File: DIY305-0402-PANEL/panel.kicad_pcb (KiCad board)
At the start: 2 copper layers, 45.2 x 39 mm, 388 parts, among them J1 Conn_01x07, J2 Conn_01x07

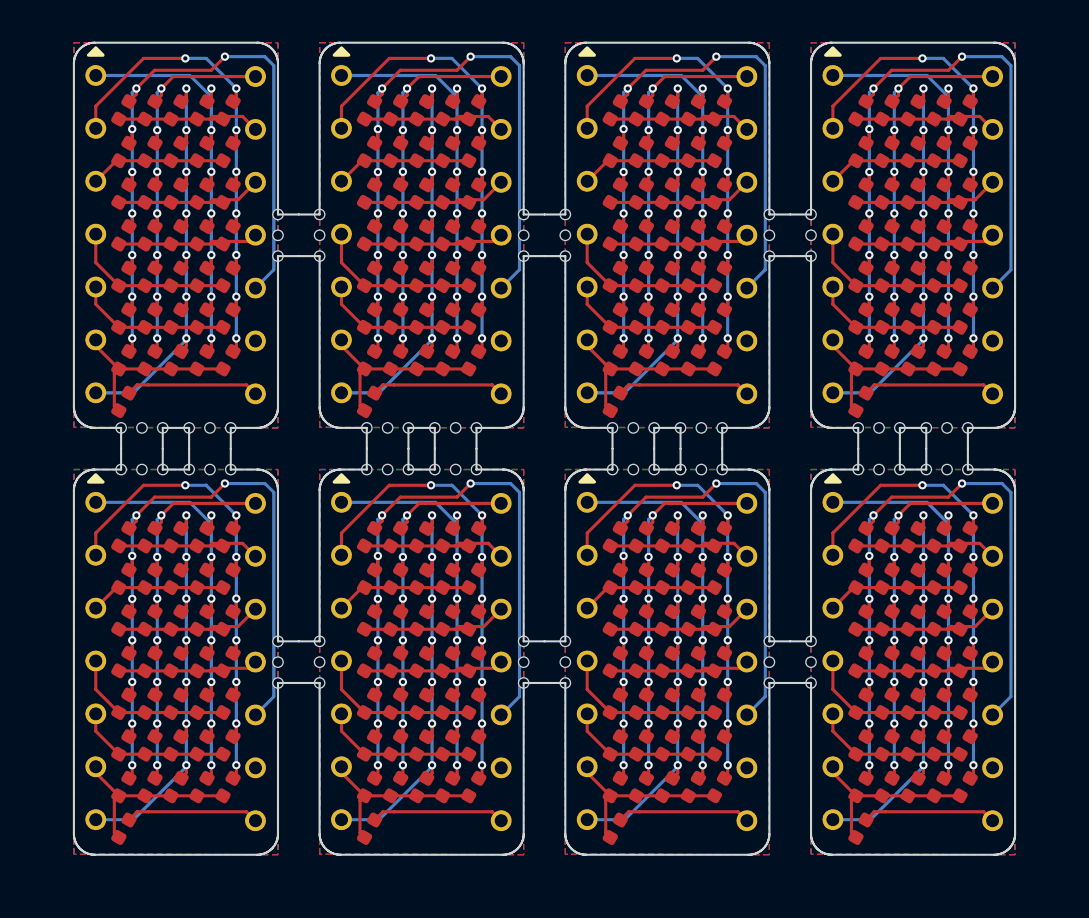
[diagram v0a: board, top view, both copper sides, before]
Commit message: Added pannel
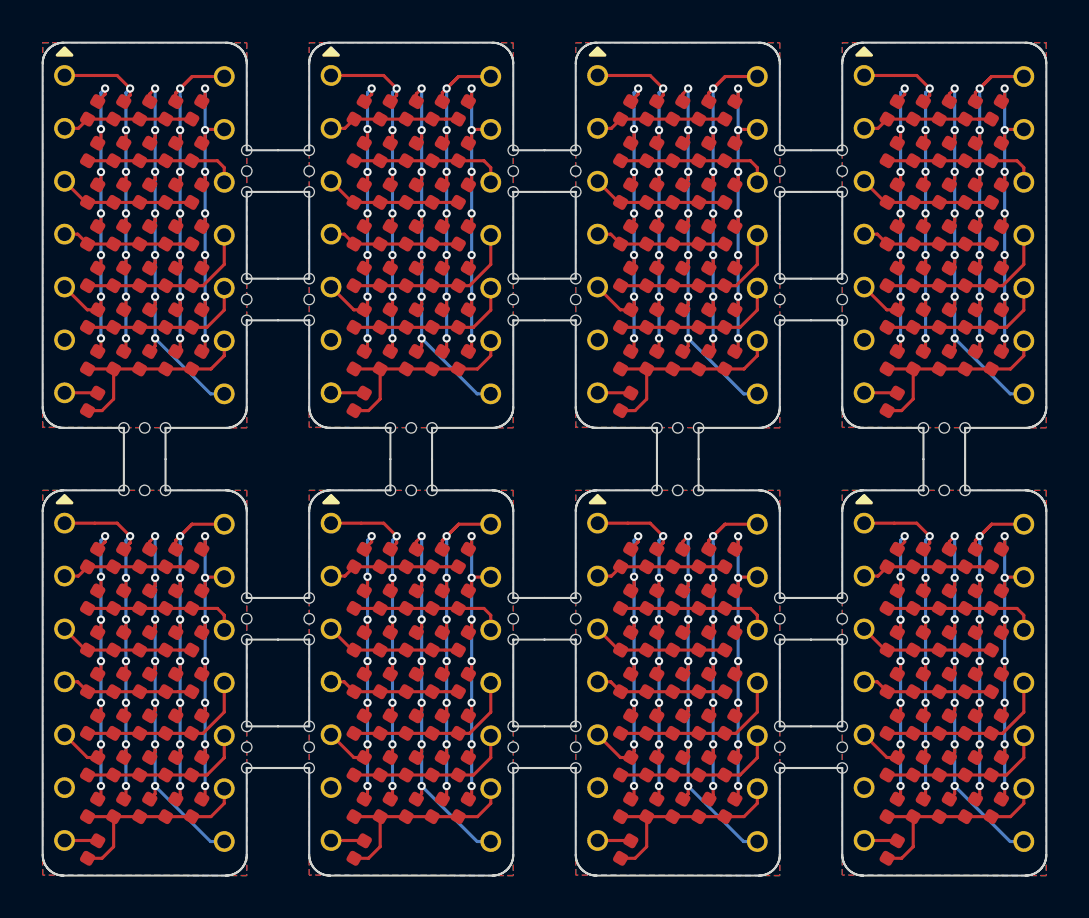
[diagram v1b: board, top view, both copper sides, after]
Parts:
- removed the D1 at (128.3, 23.2)
- removed the D1 at (128.3, 43.8)
- removed the D1 at (140.1, 23.2)
- removed the D1 at (151.9, 23.2)
- removed the D1 at (163.7, 43.8)
- removed the D1 at (163.7, 23.2)
- removed the D1 at (140.1, 43.8)
- removed the D1 at (151.9, 43.8)
- removed the D10 at (141.3, 27.2)
- removed the D10 at (164.9, 47.8)
- removed the D10 at (129.6, 47.8)
- removed the D10 at (129.6, 27.2)
- removed the D10 at (153.2, 27.2)
- removed the D10 at (153.2, 47.8)
- removed the D10 at (141.3, 47.8)
- removed the D10 at (164.9, 27.2)
- removed the D11 at (153.2, 29.2)
- removed the D11 at (129.6, 49.8)
- removed the D11 at (153.2, 49.8)
- removed the D11 at (141.3, 49.8)
- removed the D11 at (141.3, 29.2)
- removed the D11 at (164.9, 29.2)
- removed the D11 at (164.9, 49.8)
- removed the D11 at (129.6, 29.2)
- removed the D12 at (153.2, 31.2)
- removed the D12 at (164.9, 31.2)
- removed the D12 at (141.3, 31.2)
- removed the D12 at (129.6, 51.8)
- removed the D12 at (164.9, 51.8)
- removed the D12 at (129.6, 31.2)
- removed the D12 at (153.2, 51.8)
- removed the D12 at (141.3, 51.8)
- removed the D13 at (141.3, 33.2)
- removed the D13 at (164.9, 53.8)
- removed the D13 at (164.9, 33.2)
- removed the D13 at (129.6, 53.8)
- removed the D13 at (141.3, 53.8)
- removed the D13 at (153.2, 53.8)
- removed the D13 at (153.2, 33.2)
- removed the D13 at (129.6, 33.2)
- removed the D14 at (164.9, 55.8)
- removed the D14 at (164.9, 35.2)
- removed the D14 at (153.2, 35.2)
- removed the D14 at (141.3, 35.2)
- removed the D14 at (129.6, 55.8)
- removed the D14 at (129.6, 35.2)
- removed the D14 at (141.3, 55.8)
- removed the D14 at (153.2, 55.8)
- removed the D15 at (130.8, 23.2)
- removed the D15 at (166.2, 43.8)
- removed the D15 at (130.8, 43.8)
- removed the D15 at (166.2, 23.2)
- removed the D15 at (154.4, 43.8)
- removed the D15 at (142.6, 43.8)
- removed the D15 at (154.4, 23.2)
- removed the D15 at (142.6, 23.2)
- removed the D16 at (142.6, 25.2)
- removed the D16 at (154.4, 25.2)
- removed the D16 at (166.2, 45.8)
- removed the D16 at (142.6, 45.8)
- removed the D16 at (166.2, 25.2)
- removed the D16 at (130.8, 45.8)
- removed the D16 at (130.8, 25.2)
- removed the D16 at (154.4, 45.8)
- removed the D17 at (142.6, 47.8)
- removed the D17 at (130.8, 47.8)
- removed the D17 at (130.8, 27.2)
- removed the D17 at (154.4, 47.8)
- removed the D17 at (154.4, 27.2)
- removed the D17 at (166.2, 27.2)
- removed the D17 at (166.2, 47.8)
- removed the D17 at (142.6, 27.2)
- removed the D18 at (154.4, 29.2)
- removed the D18 at (142.6, 29.2)
- removed the D18 at (154.4, 49.8)
- removed the D18 at (166.2, 29.2)
- removed the D18 at (130.8, 29.2)
- removed the D18 at (166.2, 49.8)
- removed the D18 at (130.8, 49.8)
- removed the D18 at (142.6, 49.8)
- removed the D19 at (166.2, 31.2)
- removed the D19 at (154.4, 31.2)
- removed the D19 at (154.4, 51.8)
- removed the D19 at (142.6, 31.2)
- removed the D19 at (130.8, 51.8)
- removed the D19 at (130.8, 31.2)
- removed the D19 at (166.2, 51.8)
- removed the D19 at (142.6, 51.8)
- removed the D2 at (151.9, 45.8)
- removed the D2 at (128.3, 45.8)
- removed the D2 at (163.7, 45.8)
- removed the D2 at (163.7, 25.2)
- removed the D2 at (140.1, 25.2)
- removed the D2 at (140.1, 45.8)
- removed the D2 at (151.9, 25.2)
- removed the D2 at (128.3, 25.2)
- removed the D20 at (154.4, 33.2)
- removed the D20 at (166.2, 33.2)
- removed the D20 at (142.6, 53.8)
- removed the D20 at (130.8, 53.8)
- removed the D20 at (154.4, 53.8)
- removed the D20 at (130.8, 33.2)
- removed the D20 at (166.2, 53.8)
- removed the D20 at (142.6, 33.2)
- removed the D21 at (142.6, 35.2)
- removed the D21 at (166.2, 35.2)
- removed the D21 at (166.2, 55.8)
- removed the D21 at (154.4, 35.2)
- removed the D21 at (130.8, 55.8)
- removed the D21 at (154.4, 55.8)
- removed the D21 at (130.8, 35.2)
- removed the D21 at (142.6, 55.8)
- removed the D22 at (143.8, 43.8)
- removed the D22 at (143.8, 23.2)
- removed the D22 at (132.1, 43.8)
- removed the D22 at (167.4, 23.2)
- removed the D22 at (155.7, 43.8)
- removed the D22 at (155.7, 23.2)
- removed the D22 at (132.1, 23.2)
- removed the D22 at (167.4, 43.8)
- removed the D23 at (132.1, 45.8)
- removed the D23 at (167.4, 25.2)
- removed the D23 at (132.1, 25.2)
- removed the D23 at (155.7, 45.8)
- removed the D23 at (155.7, 25.2)
- removed the D23 at (143.8, 45.8)
- removed the D23 at (143.8, 25.2)
- removed the D23 at (167.4, 45.8)
- removed the D24 at (167.4, 47.8)
- removed the D24 at (155.7, 27.2)
- removed the D24 at (143.8, 47.8)
- removed the D24 at (167.4, 27.2)
- removed the D24 at (132.1, 27.2)
- removed the D24 at (155.7, 47.8)
- removed the D24 at (143.8, 27.2)
- removed the D24 at (132.1, 47.8)
- removed the D25 at (167.4, 49.8)
- removed the D25 at (155.7, 49.8)
- removed the D25 at (143.8, 29.2)
- removed the D25 at (155.7, 29.2)
- removed the D25 at (132.1, 49.8)
- removed the D25 at (132.1, 29.2)
- removed the D25 at (167.4, 29.2)
- removed the D25 at (143.8, 49.8)
- removed the D26 at (132.1, 31.2)
- removed the D26 at (155.7, 31.2)
- removed the D26 at (155.7, 51.8)
- removed the D26 at (143.8, 51.8)
- removed the D26 at (167.4, 51.8)
- removed the D26 at (167.4, 31.2)
- removed the D26 at (143.8, 31.2)
- removed the D26 at (132.1, 51.8)
- removed the D27 at (155.7, 53.8)
- removed the D27 at (155.7, 33.2)
- removed the D27 at (132.1, 53.8)
- removed the D27 at (143.8, 33.2)
- removed the D27 at (132.1, 33.2)
- removed the D27 at (167.4, 53.8)
- removed the D27 at (167.4, 33.2)
- removed the D27 at (143.8, 53.8)
- removed the D28 at (167.4, 35.2)
- removed the D28 at (143.8, 35.2)
- removed the D28 at (132.1, 55.8)
- removed the D28 at (167.4, 55.8)
- removed the D28 at (155.7, 35.2)
- removed the D28 at (155.7, 55.8)
- removed the D28 at (132.1, 35.2)
- removed the D28 at (143.8, 55.8)
- removed the D29 at (133.3, 43.8)
- removed the D29 at (156.9, 23.2)
- removed the D29 at (168.7, 43.8)
- removed the D29 at (145.1, 23.2)
- removed the D29 at (168.7, 23.2)
- removed the D29 at (145.1, 43.8)
- removed the D29 at (156.9, 43.8)
- removed the D29 at (133.3, 23.2)
- removed the D3 at (128.3, 27.2)
- removed the D3 at (140.1, 27.2)
- removed the D3 at (151.9, 27.2)
- removed the D3 at (163.7, 27.2)
- removed the D3 at (128.3, 47.8)
- removed the D3 at (140.1, 47.8)
- removed the D3 at (151.9, 47.8)
- removed the D3 at (163.7, 47.8)
- removed the D30 at (133.3, 45.8)
- removed the D30 at (145.1, 45.8)
- removed the D30 at (156.9, 45.8)
- removed the D30 at (156.9, 25.2)
- removed the D30 at (133.3, 25.2)
- removed the D30 at (168.7, 25.2)
- removed the D30 at (145.1, 25.2)
- removed the D30 at (168.7, 45.8)
- removed the D31 at (145.1, 27.2)
- removed the D31 at (133.3, 27.2)
- removed the D31 at (156.9, 27.2)
- removed the D31 at (168.7, 47.8)
- removed the D31 at (168.7, 27.2)
- removed the D31 at (156.9, 47.8)
- removed the D31 at (145.1, 47.8)
- removed the D31 at (133.3, 47.8)
- removed the D32 at (145.1, 29.2)
- removed the D32 at (145.1, 49.8)
- removed the D32 at (168.7, 29.2)
- removed the D32 at (156.9, 49.8)
- removed the D32 at (133.3, 29.2)
- removed the D32 at (156.9, 29.2)
- removed the D32 at (133.3, 49.8)
- removed the D32 at (168.7, 49.8)
- removed the D33 at (145.1, 51.8)
- removed the D33 at (156.9, 31.2)
- removed the D33 at (145.1, 31.2)
- removed the D33 at (133.3, 31.2)
- removed the D33 at (133.3, 51.8)
- removed the D33 at (168.7, 51.8)
- removed the D33 at (168.7, 31.2)
- removed the D33 at (156.9, 51.8)
- removed the D34 at (145.1, 53.8)
- removed the D34 at (156.9, 33.2)
- removed the D34 at (133.3, 53.8)
- removed the D34 at (168.7, 33.2)
- removed the D34 at (168.7, 53.8)
- removed the D34 at (133.3, 33.2)
- removed the D34 at (145.1, 33.2)
- removed the D34 at (156.9, 53.8)
- removed the D35 at (145.1, 35.2)
- removed the D35 at (156.9, 35.2)
- removed the D35 at (168.7, 55.8)
- removed the D35 at (145.1, 55.8)
- removed the D35 at (133.3, 35.2)
- removed the D35 at (133.3, 55.8)
- removed the D35 at (168.7, 35.2)
- removed the D35 at (156.9, 55.8)
- removed the D36 at (140.1, 37.2)
- removed the D36 at (163.7, 37.2)
- removed the D36 at (140.1, 57.8)
- removed the D36 at (128.3, 37.2)
- removed the D36 at (128.3, 57.8)
- removed the D36 at (151.9, 57.8)
- removed the D36 at (151.9, 37.2)
- removed the D36 at (163.7, 57.8)
- removed the D4 at (128.3, 29.2)
- removed the D4 at (140.1, 29.2)
- removed the D4 at (163.7, 49.8)
- removed the D4 at (163.7, 29.2)
- removed the D4 at (140.1, 49.8)
- removed the D4 at (151.9, 49.8)
- removed the D4 at (151.9, 29.2)
- removed the D4 at (128.3, 49.8)
- removed the D5 at (140.1, 51.8)
- removed the D5 at (128.3, 31.2)
- removed the D5 at (151.9, 51.8)
- removed the D5 at (151.9, 31.2)
- removed the D5 at (128.3, 51.8)
- removed the D5 at (163.7, 31.2)
- removed the D5 at (163.7, 51.8)
- removed the D5 at (140.1, 31.2)
- removed the D6 at (163.7, 33.2)
- removed the D6 at (163.7, 53.8)
- removed the D6 at (151.9, 53.8)
- removed the D6 at (128.3, 53.8)
- removed the D6 at (140.1, 53.8)
- removed the D6 at (140.1, 33.2)
- removed the D6 at (128.3, 33.2)
- removed the D6 at (151.9, 33.2)
- removed the D7 at (128.3, 35.2)
- removed the D7 at (163.7, 55.8)
- removed the D7 at (128.3, 55.8)
- removed the D7 at (140.1, 35.2)
- removed the D7 at (151.9, 35.2)
- removed the D7 at (163.7, 35.2)
- removed the D7 at (151.9, 55.8)
- removed the D7 at (140.1, 55.8)
- removed the D8 at (164.9, 23.2)
- removed the D8 at (153.2, 43.8)
- removed the D8 at (129.6, 23.2)
- removed the D8 at (153.2, 23.2)
- removed the D8 at (141.3, 23.2)
- removed the D8 at (141.3, 43.8)
- removed the D8 at (164.9, 43.8)
- removed the D8 at (129.6, 43.8)
- removed the D9 at (141.3, 25.2)
- removed the D9 at (164.9, 25.2)
- removed the D9 at (141.3, 45.8)
- removed the D9 at (153.2, 25.2)
- removed the D9 at (153.2, 45.8)
- removed the D9 at (129.6, 25.2)
- removed the D9 at (164.9, 45.8)
- removed the D9 at (129.6, 45.8)
- removed the J1 at (127.0, 21.6)
- removed the J1 at (138.8, 42.1)
- removed the J1 at (127.0, 42.1)
- removed the J1 at (162.3, 42.1)
- removed the J1 at (150.6, 21.6)
- removed the J1 at (162.3, 21.6)
- removed the J1 at (150.6, 42.1)
- removed the J1 at (138.8, 21.6)
- removed the J2 at (158.2, 21.6)
- removed the J2 at (158.2, 42.1)
- removed the J2 at (146.4, 21.6)
- removed the J2 at (134.6, 42.1)
- removed the J2 at (146.4, 42.1)
- removed the J2 at (170.0, 42.1)
- removed the J2 at (134.6, 21.6)
- removed the J2 at (170.0, 21.6)
- removed REF** (x84): NPTH, NPTH
- added D1: LED, LED_SMD:LED_0402_1005Metric, F.Cu at (152.4, 44.8)
- added D1: LED, LED_SMD:LED_0402_1005Metric, F.Cu at (152.4, 23.2)
- added D1: LED, LED_SMD:LED_0402_1005Metric, F.Cu at (139.6, 23.2)
- added D1: LED, LED_SMD:LED_0402_1005Metric, F.Cu at (126.8, 44.8)
- added D1: LED, LED_SMD:LED_0402_1005Metric, F.Cu at (165.2, 44.8)
- added D1: LED, LED_SMD:LED_0402_1005Metric, F.Cu at (126.8, 23.2)
- added D1: LED, LED_SMD:LED_0402_1005Metric, F.Cu at (139.6, 44.8)
- added D1: LED, LED_SMD:LED_0402_1005Metric, F.Cu at (165.2, 23.2)
- added D10: LED, LED_SMD:LED_0402_1005Metric, F.Cu at (140.8, 48.8)
- added D10: LED, LED_SMD:LED_0402_1005Metric, F.Cu at (128.1, 48.8)
- added D10: LED, LED_SMD:LED_0402_1005Metric, F.Cu at (166.4, 27.2)
- added D10: LED, LED_SMD:LED_0402_1005Metric, F.Cu at (140.8, 27.2)
- added D10: LED, LED_SMD:LED_0402_1005Metric, F.Cu at (166.4, 48.8)
- added D10: LED, LED_SMD:LED_0402_1005Metric, F.Cu at (153.7, 48.8)
- added D10: LED, LED_SMD:LED_0402_1005Metric, F.Cu at (153.7, 27.2)
- added D10: LED, LED_SMD:LED_0402_1005Metric, F.Cu at (128.1, 27.2)
- added D11: LED, LED_SMD:LED_0402_1005Metric, F.Cu at (166.4, 29.2)
- added D11: LED, LED_SMD:LED_0402_1005Metric, F.Cu at (153.7, 50.8)
- added D11: LED, LED_SMD:LED_0402_1005Metric, F.Cu at (140.8, 29.2)
- added D11: LED, LED_SMD:LED_0402_1005Metric, F.Cu at (128.1, 50.8)
- added D11: LED, LED_SMD:LED_0402_1005Metric, F.Cu at (128.1, 29.2)
- added D11: LED, LED_SMD:LED_0402_1005Metric, F.Cu at (140.8, 50.8)
- added D11: LED, LED_SMD:LED_0402_1005Metric, F.Cu at (153.7, 29.2)
- added D11: LED, LED_SMD:LED_0402_1005Metric, F.Cu at (166.4, 50.8)
- added D12: LED, LED_SMD:LED_0402_1005Metric, F.Cu at (166.4, 31.2)
- added D12: LED, LED_SMD:LED_0402_1005Metric, F.Cu at (128.1, 31.2)
- added D12: LED, LED_SMD:LED_0402_1005Metric, F.Cu at (128.1, 52.8)
- added D12: LED, LED_SMD:LED_0402_1005Metric, F.Cu at (140.8, 31.2)
- added D12: LED, LED_SMD:LED_0402_1005Metric, F.Cu at (140.8, 52.8)
- added D12: LED, LED_SMD:LED_0402_1005Metric, F.Cu at (166.4, 52.8)
- added D12: LED, LED_SMD:LED_0402_1005Metric, F.Cu at (153.7, 52.8)
- added D12: LED, LED_SMD:LED_0402_1005Metric, F.Cu at (153.7, 31.2)
- added D13: LED, LED_SMD:LED_0402_1005Metric, F.Cu at (128.1, 33.2)
- added D13: LED, LED_SMD:LED_0402_1005Metric, F.Cu at (166.4, 33.2)
- added D13: LED, LED_SMD:LED_0402_1005Metric, F.Cu at (128.1, 54.8)
- added D13: LED, LED_SMD:LED_0402_1005Metric, F.Cu at (153.7, 54.8)
- added D13: LED, LED_SMD:LED_0402_1005Metric, F.Cu at (166.4, 54.8)
- added D13: LED, LED_SMD:LED_0402_1005Metric, F.Cu at (140.8, 54.8)
- added D13: LED, LED_SMD:LED_0402_1005Metric, F.Cu at (153.7, 33.2)
- added D13: LED, LED_SMD:LED_0402_1005Metric, F.Cu at (140.8, 33.2)
- added D14: LED, LED_SMD:LED_0402_1005Metric, F.Cu at (128.1, 56.8)
- added D14: LED, LED_SMD:LED_0402_1005Metric, F.Cu at (140.8, 56.8)
- added D14: LED, LED_SMD:LED_0402_1005Metric, F.Cu at (166.4, 35.2)
- added D14: LED, LED_SMD:LED_0402_1005Metric, F.Cu at (153.7, 56.8)
- added D14: LED, LED_SMD:LED_0402_1005Metric, F.Cu at (166.4, 56.8)
- added D14: LED, LED_SMD:LED_0402_1005Metric, F.Cu at (140.8, 35.2)
- added D14: LED, LED_SMD:LED_0402_1005Metric, F.Cu at (153.7, 35.2)
- added D14: LED, LED_SMD:LED_0402_1005Metric, F.Cu at (128.1, 35.2)
- added D15: LED, LED_SMD:LED_0402_1005Metric, F.Cu at (142.1, 44.8)
- added D15: LED, LED_SMD:LED_0402_1005Metric, F.Cu at (142.1, 23.2)
- added D15: LED, LED_SMD:LED_0402_1005Metric, F.Cu at (167.7, 44.8)
- added D15: LED, LED_SMD:LED_0402_1005Metric, F.Cu at (167.7, 23.2)
- added D15: LED, LED_SMD:LED_0402_1005Metric, F.Cu at (154.9, 44.8)
- added D15: LED, LED_SMD:LED_0402_1005Metric, F.Cu at (129.3, 23.2)
- added D15: LED, LED_SMD:LED_0402_1005Metric, F.Cu at (129.3, 44.8)
- added D15: LED, LED_SMD:LED_0402_1005Metric, F.Cu at (154.9, 23.2)
- added D16: LED, LED_SMD:LED_0402_1005Metric, F.Cu at (167.7, 46.8)
- added D16: LED, LED_SMD:LED_0402_1005Metric, F.Cu at (129.3, 46.8)
- added D16: LED, LED_SMD:LED_0402_1005Metric, F.Cu at (142.1, 25.2)
- added D16: LED, LED_SMD:LED_0402_1005Metric, F.Cu at (142.1, 46.8)
- added D16: LED, LED_SMD:LED_0402_1005Metric, F.Cu at (154.9, 46.8)
- added D16: LED, LED_SMD:LED_0402_1005Metric, F.Cu at (129.3, 25.2)
- added D16: LED, LED_SMD:LED_0402_1005Metric, F.Cu at (167.7, 25.2)
- added D16: LED, LED_SMD:LED_0402_1005Metric, F.Cu at (154.9, 25.2)
- added D17: LED, LED_SMD:LED_0402_1005Metric, F.Cu at (129.3, 48.8)
- added D17: LED, LED_SMD:LED_0402_1005Metric, F.Cu at (129.3, 27.2)
- added D17: LED, LED_SMD:LED_0402_1005Metric, F.Cu at (154.9, 48.8)
- added D17: LED, LED_SMD:LED_0402_1005Metric, F.Cu at (167.7, 27.2)
- added D17: LED, LED_SMD:LED_0402_1005Metric, F.Cu at (154.9, 27.2)
- added D17: LED, LED_SMD:LED_0402_1005Metric, F.Cu at (167.7, 48.8)
- added D17: LED, LED_SMD:LED_0402_1005Metric, F.Cu at (142.1, 27.2)
- added D17: LED, LED_SMD:LED_0402_1005Metric, F.Cu at (142.1, 48.8)
- added D18: LED, LED_SMD:LED_0402_1005Metric, F.Cu at (167.7, 50.8)
- added D18: LED, LED_SMD:LED_0402_1005Metric, F.Cu at (154.9, 50.8)
- added D18: LED, LED_SMD:LED_0402_1005Metric, F.Cu at (167.7, 29.2)
- added D18: LED, LED_SMD:LED_0402_1005Metric, F.Cu at (129.3, 50.8)
- added D18: LED, LED_SMD:LED_0402_1005Metric, F.Cu at (142.1, 29.2)
- added D18: LED, LED_SMD:LED_0402_1005Metric, F.Cu at (142.1, 50.8)
- added D18: LED, LED_SMD:LED_0402_1005Metric, F.Cu at (154.9, 29.2)
- added D18: LED, LED_SMD:LED_0402_1005Metric, F.Cu at (129.3, 29.2)
- added D19: LED, LED_SMD:LED_0402_1005Metric, F.Cu at (129.3, 31.2)
- added D19: LED, LED_SMD:LED_0402_1005Metric, F.Cu at (167.7, 31.2)
- added D19: LED, LED_SMD:LED_0402_1005Metric, F.Cu at (142.1, 52.8)
- added D19: LED, LED_SMD:LED_0402_1005Metric, F.Cu at (142.1, 31.2)
- added D19: LED, LED_SMD:LED_0402_1005Metric, F.Cu at (154.9, 52.8)
- added D19: LED, LED_SMD:LED_0402_1005Metric, F.Cu at (154.9, 31.2)
- added D19: LED, LED_SMD:LED_0402_1005Metric, F.Cu at (167.7, 52.8)
- added D19: LED, LED_SMD:LED_0402_1005Metric, F.Cu at (129.3, 52.8)
- added D2: LED, LED_SMD:LED_0402_1005Metric, F.Cu at (165.2, 46.8)
- added D2: LED, LED_SMD:LED_0402_1005Metric, F.Cu at (126.8, 46.8)
- added D2: LED, LED_SMD:LED_0402_1005Metric, F.Cu at (126.8, 25.2)
- added D2: LED, LED_SMD:LED_0402_1005Metric, F.Cu at (139.6, 46.8)
- added D2: LED, LED_SMD:LED_0402_1005Metric, F.Cu at (165.2, 25.2)
- added D2: LED, LED_SMD:LED_0402_1005Metric, F.Cu at (139.6, 25.2)
- added D2: LED, LED_SMD:LED_0402_1005Metric, F.Cu at (152.4, 25.2)
- added D2: LED, LED_SMD:LED_0402_1005Metric, F.Cu at (152.4, 46.8)
- added D20: LED, LED_SMD:LED_0402_1005Metric, F.Cu at (142.1, 54.8)
- added D20: LED, LED_SMD:LED_0402_1005Metric, F.Cu at (154.9, 33.2)
- added D20: LED, LED_SMD:LED_0402_1005Metric, F.Cu at (129.3, 33.2)
- added D20: LED, LED_SMD:LED_0402_1005Metric, F.Cu at (154.9, 54.8)
- added D20: LED, LED_SMD:LED_0402_1005Metric, F.Cu at (167.7, 33.2)
- added D20: LED, LED_SMD:LED_0402_1005Metric, F.Cu at (142.1, 33.2)
- added D20: LED, LED_SMD:LED_0402_1005Metric, F.Cu at (167.7, 54.8)
- added D20: LED, LED_SMD:LED_0402_1005Metric, F.Cu at (129.3, 54.8)
- added D21: LED, LED_SMD:LED_0402_1005Metric, F.Cu at (129.3, 35.2)
- added D21: LED, LED_SMD:LED_0402_1005Metric, F.Cu at (154.9, 35.2)
- added D21: LED, LED_SMD:LED_0402_1005Metric, F.Cu at (154.9, 56.8)
- added D21: LED, LED_SMD:LED_0402_1005Metric, F.Cu at (142.1, 56.8)
- added D21: LED, LED_SMD:LED_0402_1005Metric, F.Cu at (129.3, 56.8)
- added D21: LED, LED_SMD:LED_0402_1005Metric, F.Cu at (167.7, 56.8)
- added D21: LED, LED_SMD:LED_0402_1005Metric, F.Cu at (167.7, 35.2)
- added D21: LED, LED_SMD:LED_0402_1005Metric, F.Cu at (142.1, 35.2)
- added D22: LED, LED_SMD:LED_0402_1005Metric, F.Cu at (143.3, 44.8)
- added D22: LED, LED_SMD:LED_0402_1005Metric, F.Cu at (130.6, 44.8)
- added D22: LED, LED_SMD:LED_0402_1005Metric, F.Cu at (156.2, 44.8)
- added D22: LED, LED_SMD:LED_0402_1005Metric, F.Cu at (156.2, 23.2)
- added D22: LED, LED_SMD:LED_0402_1005Metric, F.Cu at (143.3, 23.2)
- added D22: LED, LED_SMD:LED_0402_1005Metric, F.Cu at (130.6, 23.2)
- added D22: LED, LED_SMD:LED_0402_1005Metric, F.Cu at (168.9, 23.2)
- added D22: LED, LED_SMD:LED_0402_1005Metric, F.Cu at (168.9, 44.8)
- added D23: LED, LED_SMD:LED_0402_1005Metric, F.Cu at (143.3, 25.2)
- added D23: LED, LED_SMD:LED_0402_1005Metric, F.Cu at (130.6, 25.2)
- added D23: LED, LED_SMD:LED_0402_1005Metric, F.Cu at (168.9, 25.2)
- added D23: LED, LED_SMD:LED_0402_1005Metric, F.Cu at (156.2, 46.8)
- added D23: LED, LED_SMD:LED_0402_1005Metric, F.Cu at (168.9, 46.8)
- added D23: LED, LED_SMD:LED_0402_1005Metric, F.Cu at (156.2, 25.2)
- added D23: LED, LED_SMD:LED_0402_1005Metric, F.Cu at (143.3, 46.8)
- added D23: LED, LED_SMD:LED_0402_1005Metric, F.Cu at (130.6, 46.8)
- added D24: LED, LED_SMD:LED_0402_1005Metric, F.Cu at (130.6, 27.2)
- added D24: LED, LED_SMD:LED_0402_1005Metric, F.Cu at (156.2, 27.2)
- added D24: LED, LED_SMD:LED_0402_1005Metric, F.Cu at (143.3, 27.2)
- added D24: LED, LED_SMD:LED_0402_1005Metric, F.Cu at (168.9, 27.2)
- added D24: LED, LED_SMD:LED_0402_1005Metric, F.Cu at (156.2, 48.8)
- added D24: LED, LED_SMD:LED_0402_1005Metric, F.Cu at (143.3, 48.8)
- added D24: LED, LED_SMD:LED_0402_1005Metric, F.Cu at (168.9, 48.8)
- added D24: LED, LED_SMD:LED_0402_1005Metric, F.Cu at (130.6, 48.8)
- added D25: LED, LED_SMD:LED_0402_1005Metric, F.Cu at (130.6, 50.8)
- added D25: LED, LED_SMD:LED_0402_1005Metric, F.Cu at (168.9, 29.2)
- added D25: LED, LED_SMD:LED_0402_1005Metric, F.Cu at (156.2, 29.2)
- added D25: LED, LED_SMD:LED_0402_1005Metric, F.Cu at (168.9, 50.8)
- added D25: LED, LED_SMD:LED_0402_1005Metric, F.Cu at (130.6, 29.2)
- added D25: LED, LED_SMD:LED_0402_1005Metric, F.Cu at (156.2, 50.8)
- added D25: LED, LED_SMD:LED_0402_1005Metric, F.Cu at (143.3, 29.2)
- added D25: LED, LED_SMD:LED_0402_1005Metric, F.Cu at (143.3, 50.8)
- added D26: LED, LED_SMD:LED_0402_1005Metric, F.Cu at (130.6, 52.8)
- added D26: LED, LED_SMD:LED_0402_1005Metric, F.Cu at (143.3, 31.2)
- added D26: LED, LED_SMD:LED_0402_1005Metric, F.Cu at (168.9, 31.2)
- added D26: LED, LED_SMD:LED_0402_1005Metric, F.Cu at (143.3, 52.8)
- added D26: LED, LED_SMD:LED_0402_1005Metric, F.Cu at (156.2, 52.8)
- added D26: LED, LED_SMD:LED_0402_1005Metric, F.Cu at (156.2, 31.2)
- added D26: LED, LED_SMD:LED_0402_1005Metric, F.Cu at (130.6, 31.2)
- added D26: LED, LED_SMD:LED_0402_1005Metric, F.Cu at (168.9, 52.8)
- added D27: LED, LED_SMD:LED_0402_1005Metric, F.Cu at (143.3, 33.2)
- added D27: LED, LED_SMD:LED_0402_1005Metric, F.Cu at (156.2, 54.8)
- added D27: LED, LED_SMD:LED_0402_1005Metric, F.Cu at (130.6, 54.8)
- added D27: LED, LED_SMD:LED_0402_1005Metric, F.Cu at (143.3, 54.8)
- added D27: LED, LED_SMD:LED_0402_1005Metric, F.Cu at (168.9, 54.8)
- added D27: LED, LED_SMD:LED_0402_1005Metric, F.Cu at (168.9, 33.2)
- added D27: LED, LED_SMD:LED_0402_1005Metric, F.Cu at (130.6, 33.2)
- added D27: LED, LED_SMD:LED_0402_1005Metric, F.Cu at (156.2, 33.2)
- added D28: LED, LED_SMD:LED_0402_1005Metric, F.Cu at (168.9, 56.8)
- added D28: LED, LED_SMD:LED_0402_1005Metric, F.Cu at (168.9, 35.2)
- added D28: LED, LED_SMD:LED_0402_1005Metric, F.Cu at (156.2, 56.8)
- added D28: LED, LED_SMD:LED_0402_1005Metric, F.Cu at (156.2, 35.2)
- added D28: LED, LED_SMD:LED_0402_1005Metric, F.Cu at (130.6, 35.2)
- added D28: LED, LED_SMD:LED_0402_1005Metric, F.Cu at (143.3, 56.8)
- added D28: LED, LED_SMD:LED_0402_1005Metric, F.Cu at (143.3, 35.2)
- added D28: LED, LED_SMD:LED_0402_1005Metric, F.Cu at (130.6, 56.8)
- added D29: LED, LED_SMD:LED_0402_1005Metric, F.Cu at (157.4, 23.2)
- added D29: LED, LED_SMD:LED_0402_1005Metric, F.Cu at (157.4, 44.8)
- added D29: LED, LED_SMD:LED_0402_1005Metric, F.Cu at (170.2, 44.8)
- added D29: LED, LED_SMD:LED_0402_1005Metric, F.Cu at (131.8, 44.8)
- added D29: LED, LED_SMD:LED_0402_1005Metric, F.Cu at (144.6, 23.2)
- added D29: LED, LED_SMD:LED_0402_1005Metric, F.Cu at (131.8, 23.2)
- added D29: LED, LED_SMD:LED_0402_1005Metric, F.Cu at (144.6, 44.8)
- added D29: LED, LED_SMD:LED_0402_1005Metric, F.Cu at (170.2, 23.2)
- added D3: LED, LED_SMD:LED_0402_1005Metric, F.Cu at (139.6, 27.2)
- added D3: LED, LED_SMD:LED_0402_1005Metric, F.Cu at (165.2, 48.8)
- added D3: LED, LED_SMD:LED_0402_1005Metric, F.Cu at (152.4, 48.8)
- added D3: LED, LED_SMD:LED_0402_1005Metric, F.Cu at (126.8, 48.8)
- added D3: LED, LED_SMD:LED_0402_1005Metric, F.Cu at (126.8, 27.2)
- added D3: LED, LED_SMD:LED_0402_1005Metric, F.Cu at (139.6, 48.8)
- added D3: LED, LED_SMD:LED_0402_1005Metric, F.Cu at (152.4, 27.2)
- added D3: LED, LED_SMD:LED_0402_1005Metric, F.Cu at (165.2, 27.2)
- added D30: LED, LED_SMD:LED_0402_1005Metric, F.Cu at (170.2, 25.2)
- added D30: LED, LED_SMD:LED_0402_1005Metric, F.Cu at (131.8, 25.2)
- added D30: LED, LED_SMD:LED_0402_1005Metric, F.Cu at (157.4, 46.8)
- added D30: LED, LED_SMD:LED_0402_1005Metric, F.Cu at (131.8, 46.8)
- added D30: LED, LED_SMD:LED_0402_1005Metric, F.Cu at (170.2, 46.8)
- added D30: LED, LED_SMD:LED_0402_1005Metric, F.Cu at (144.6, 25.2)
- added D30: LED, LED_SMD:LED_0402_1005Metric, F.Cu at (157.4, 25.2)
- added D30: LED, LED_SMD:LED_0402_1005Metric, F.Cu at (144.6, 46.8)
- added D31: LED, LED_SMD:LED_0402_1005Metric, F.Cu at (157.4, 27.2)
- added D31: LED, LED_SMD:LED_0402_1005Metric, F.Cu at (144.6, 48.8)
- added D31: LED, LED_SMD:LED_0402_1005Metric, F.Cu at (144.6, 27.2)
- added D31: LED, LED_SMD:LED_0402_1005Metric, F.Cu at (131.8, 27.2)
- added D31: LED, LED_SMD:LED_0402_1005Metric, F.Cu at (170.2, 27.2)
- added D31: LED, LED_SMD:LED_0402_1005Metric, F.Cu at (157.4, 48.8)
- added D31: LED, LED_SMD:LED_0402_1005Metric, F.Cu at (170.2, 48.8)
- added D31: LED, LED_SMD:LED_0402_1005Metric, F.Cu at (131.8, 48.8)
- added D32: LED, LED_SMD:LED_0402_1005Metric, F.Cu at (131.8, 29.2)
- added D32: LED, LED_SMD:LED_0402_1005Metric, F.Cu at (157.4, 29.2)
- added D32: LED, LED_SMD:LED_0402_1005Metric, F.Cu at (144.6, 50.8)
- added D32: LED, LED_SMD:LED_0402_1005Metric, F.Cu at (170.2, 29.2)
- added D32: LED, LED_SMD:LED_0402_1005Metric, F.Cu at (170.2, 50.8)
- added D32: LED, LED_SMD:LED_0402_1005Metric, F.Cu at (157.4, 50.8)
- added D32: LED, LED_SMD:LED_0402_1005Metric, F.Cu at (131.8, 50.8)
- added D32: LED, LED_SMD:LED_0402_1005Metric, F.Cu at (144.6, 29.2)
- added D33: LED, LED_SMD:LED_0402_1005Metric, F.Cu at (157.4, 31.2)
- added D33: LED, LED_SMD:LED_0402_1005Metric, F.Cu at (170.2, 31.2)
- added D33: LED, LED_SMD:LED_0402_1005Metric, F.Cu at (170.2, 52.8)
- added D33: LED, LED_SMD:LED_0402_1005Metric, F.Cu at (144.6, 31.2)
- added D33: LED, LED_SMD:LED_0402_1005Metric, F.Cu at (157.4, 52.8)
- added D33: LED, LED_SMD:LED_0402_1005Metric, F.Cu at (131.8, 31.2)
- added D33: LED, LED_SMD:LED_0402_1005Metric, F.Cu at (131.8, 52.8)
- added D33: LED, LED_SMD:LED_0402_1005Metric, F.Cu at (144.6, 52.8)
- added D34: LED, LED_SMD:LED_0402_1005Metric, F.Cu at (131.8, 54.8)
- added D34: LED, LED_SMD:LED_0402_1005Metric, F.Cu at (170.2, 54.8)
- added D34: LED, LED_SMD:LED_0402_1005Metric, F.Cu at (131.8, 33.2)
- added D34: LED, LED_SMD:LED_0402_1005Metric, F.Cu at (170.2, 33.2)
- added D34: LED, LED_SMD:LED_0402_1005Metric, F.Cu at (144.6, 54.8)
- added D34: LED, LED_SMD:LED_0402_1005Metric, F.Cu at (157.4, 33.2)
- added D34: LED, LED_SMD:LED_0402_1005Metric, F.Cu at (144.6, 33.2)
- added D34: LED, LED_SMD:LED_0402_1005Metric, F.Cu at (157.4, 54.8)
- added D35: LED, LED_SMD:LED_0402_1005Metric, F.Cu at (131.8, 56.8)
- added D35: LED, LED_SMD:LED_0402_1005Metric, F.Cu at (170.2, 56.8)
- added D35: LED, LED_SMD:LED_0402_1005Metric, F.Cu at (144.6, 56.8)
- added D35: LED, LED_SMD:LED_0402_1005Metric, F.Cu at (157.4, 56.8)
- added D35: LED, LED_SMD:LED_0402_1005Metric, F.Cu at (170.2, 35.2)
- added D35: LED, LED_SMD:LED_0402_1005Metric, F.Cu at (157.4, 35.2)
- added D35: LED, LED_SMD:LED_0402_1005Metric, F.Cu at (131.8, 35.2)
- added D35: LED, LED_SMD:LED_0402_1005Metric, F.Cu at (144.6, 35.2)
- added D36: LED, LED_SMD:LED_0402_1005Metric, F.Cu at (139.6, 58.8)
- added D36: LED, LED_SMD:LED_0402_1005Metric, F.Cu at (165.2, 37.2)
- added D36: LED, LED_SMD:LED_0402_1005Metric, F.Cu at (126.8, 37.2)
- added D36: LED, LED_SMD:LED_0402_1005Metric, F.Cu at (152.4, 37.2)
- added D36: LED, LED_SMD:LED_0402_1005Metric, F.Cu at (126.8, 58.8)
- added D36: LED, LED_SMD:LED_0402_1005Metric, F.Cu at (139.6, 37.2)
- added D36: LED, LED_SMD:LED_0402_1005Metric, F.Cu at (152.4, 58.8)
- added D36: LED, LED_SMD:LED_0402_1005Metric, F.Cu at (165.2, 58.8)
- added D4: LED, LED_SMD:LED_0402_1005Metric, F.Cu at (165.2, 29.2)
- added D4: LED, LED_SMD:LED_0402_1005Metric, F.Cu at (139.6, 50.8)
- added D4: LED, LED_SMD:LED_0402_1005Metric, F.Cu at (139.6, 29.2)
- added D4: LED, LED_SMD:LED_0402_1005Metric, F.Cu at (152.4, 50.8)
- added D4: LED, LED_SMD:LED_0402_1005Metric, F.Cu at (165.2, 50.8)
- added D4: LED, LED_SMD:LED_0402_1005Metric, F.Cu at (126.8, 50.8)
- added D4: LED, LED_SMD:LED_0402_1005Metric, F.Cu at (152.4, 29.2)
- added D4: LED, LED_SMD:LED_0402_1005Metric, F.Cu at (126.8, 29.2)
- added D5: LED, LED_SMD:LED_0402_1005Metric, F.Cu at (152.4, 31.2)
- added D5: LED, LED_SMD:LED_0402_1005Metric, F.Cu at (139.6, 52.8)
- added D5: LED, LED_SMD:LED_0402_1005Metric, F.Cu at (152.4, 52.8)
- added D5: LED, LED_SMD:LED_0402_1005Metric, F.Cu at (126.8, 52.8)
- added D5: LED, LED_SMD:LED_0402_1005Metric, F.Cu at (165.2, 52.8)
- added D5: LED, LED_SMD:LED_0402_1005Metric, F.Cu at (165.2, 31.2)
- added D5: LED, LED_SMD:LED_0402_1005Metric, F.Cu at (126.8, 31.2)
- added D5: LED, LED_SMD:LED_0402_1005Metric, F.Cu at (139.6, 31.2)
- added D6: LED, LED_SMD:LED_0402_1005Metric, F.Cu at (126.8, 33.2)
- added D6: LED, LED_SMD:LED_0402_1005Metric, F.Cu at (139.6, 33.2)
- added D6: LED, LED_SMD:LED_0402_1005Metric, F.Cu at (152.4, 33.2)
- added D6: LED, LED_SMD:LED_0402_1005Metric, F.Cu at (165.2, 33.2)
- added D6: LED, LED_SMD:LED_0402_1005Metric, F.Cu at (152.4, 54.8)
- added D6: LED, LED_SMD:LED_0402_1005Metric, F.Cu at (126.8, 54.8)
- added D6: LED, LED_SMD:LED_0402_1005Metric, F.Cu at (165.2, 54.8)
- added D6: LED, LED_SMD:LED_0402_1005Metric, F.Cu at (139.6, 54.8)
- added D7: LED, LED_SMD:LED_0402_1005Metric, F.Cu at (152.4, 35.2)
- added D7: LED, LED_SMD:LED_0402_1005Metric, F.Cu at (165.2, 56.8)
- added D7: LED, LED_SMD:LED_0402_1005Metric, F.Cu at (139.6, 35.2)
- added D7: LED, LED_SMD:LED_0402_1005Metric, F.Cu at (152.4, 56.8)
- added D7: LED, LED_SMD:LED_0402_1005Metric, F.Cu at (126.8, 56.8)
- added D7: LED, LED_SMD:LED_0402_1005Metric, F.Cu at (139.6, 56.8)
- added D7: LED, LED_SMD:LED_0402_1005Metric, F.Cu at (165.2, 35.2)
- added D7: LED, LED_SMD:LED_0402_1005Metric, F.Cu at (126.8, 35.2)
- added D8: LED, LED_SMD:LED_0402_1005Metric, F.Cu at (128.1, 23.2)
- added D8: LED, LED_SMD:LED_0402_1005Metric, F.Cu at (153.7, 23.2)
- added D8: LED, LED_SMD:LED_0402_1005Metric, F.Cu at (153.7, 44.8)
- added D8: LED, LED_SMD:LED_0402_1005Metric, F.Cu at (140.8, 23.2)
- added D8: LED, LED_SMD:LED_0402_1005Metric, F.Cu at (128.1, 44.8)
- added D8: LED, LED_SMD:LED_0402_1005Metric, F.Cu at (140.8, 44.8)
- added D8: LED, LED_SMD:LED_0402_1005Metric, F.Cu at (166.4, 44.8)
- added D8: LED, LED_SMD:LED_0402_1005Metric, F.Cu at (166.4, 23.2)
- added D9: LED, LED_SMD:LED_0402_1005Metric, F.Cu at (166.4, 25.2)
- added D9: LED, LED_SMD:LED_0402_1005Metric, F.Cu at (140.8, 46.8)
- added D9: LED, LED_SMD:LED_0402_1005Metric, F.Cu at (128.1, 25.2)
- added D9: LED, LED_SMD:LED_0402_1005Metric, F.Cu at (140.8, 25.2)
- added D9: LED, LED_SMD:LED_0402_1005Metric, F.Cu at (153.7, 25.2)
- added D9: LED, LED_SMD:LED_0402_1005Metric, F.Cu at (128.1, 46.8)
- added D9: LED, LED_SMD:LED_0402_1005Metric, F.Cu at (166.4, 46.8)
- added D9: LED, LED_SMD:LED_0402_1005Metric, F.Cu at (153.7, 46.8)
- added J1: Conn_01x07, Connector_PinHeader_2.54mm:PinHeader_1x07_P2.54mm_Vertical, F.Cu at (133.1, 21.6)
- added J1: Conn_01x07, Connector_PinHeader_2.54mm:PinHeader_1x07_P2.54mm_Vertical, F.Cu at (171.5, 43.1)
- added J1: Conn_01x07, Connector_PinHeader_2.54mm:PinHeader_1x07_P2.54mm_Vertical, F.Cu at (171.5, 21.6)
- added J1: Conn_01x07, Connector_PinHeader_2.54mm:PinHeader_1x07_P2.54mm_Vertical, F.Cu at (158.7, 43.1)
- added J1: Conn_01x07, Connector_PinHeader_2.54mm:PinHeader_1x07_P2.54mm_Vertical, F.Cu at (145.9, 43.1)
- added J1: Conn_01x07, Connector_PinHeader_2.54mm:PinHeader_1x07_P2.54mm_Vertical, F.Cu at (158.7, 21.6)
- added J1: Conn_01x07, Connector_PinHeader_2.54mm:PinHeader_1x07_P2.54mm_Vertical, F.Cu at (145.9, 21.6)
- added J1: Conn_01x07, Connector_PinHeader_2.54mm:PinHeader_1x07_P2.54mm_Vertical, F.Cu at (133.1, 43.1)
- added J2: Conn_01x07, Connector_PinHeader_2.54mm:PinHeader_1x07_P2.54mm_Vertical, F.Cu at (163.8, 21.6)
- added J2: Conn_01x07, Connector_PinHeader_2.54mm:PinHeader_1x07_P2.54mm_Vertical, F.Cu at (125.5, 43.1)
- added J2: Conn_01x07, Connector_PinHeader_2.54mm:PinHeader_1x07_P2.54mm_Vertical, F.Cu at (138.2, 43.1)
- added J2: Conn_01x07, Connector_PinHeader_2.54mm:PinHeader_1x07_P2.54mm_Vertical, F.Cu at (151.1, 43.1)
- added J2: Conn_01x07, Connector_PinHeader_2.54mm:PinHeader_1x07_P2.54mm_Vertical, F.Cu at (151.1, 21.6)
- added J2: Conn_01x07, Connector_PinHeader_2.54mm:PinHeader_1x07_P2.54mm_Vertical, F.Cu at (125.5, 21.6)
- added J2: Conn_01x07, Connector_PinHeader_2.54mm:PinHeader_1x07_P2.54mm_Vertical, F.Cu at (163.8, 43.1)
- added J2: Conn_01x07, Connector_PinHeader_2.54mm:PinHeader_1x07_P2.54mm_Vertical, F.Cu at (138.2, 21.6)
- added KiKit_MB_10_1: NPTH, NPTH, F.Cu at (150.0, 33.3)
- added KiKit_MB_10_2: NPTH, NPTH, F.Cu at (150.0, 32.3)
- added KiKit_MB_10_3: NPTH, NPTH, F.Cu at (150.0, 31.3)
- added KiKit_MB_11_1: NPTH, NPTH, F.Cu at (159.8, 25.2)
- added KiKit_MB_11_2: NPTH, NPTH, F.Cu at (159.8, 26.2)
- added KiKit_MB_11_3: NPTH, NPTH, F.Cu at (159.8, 27.2)
- added KiKit_MB_12_1: NPTH, NPTH, F.Cu at (159.8, 31.3)
- added KiKit_MB_12_2: NPTH, NPTH, F.Cu at (159.8, 32.3)
- added KiKit_MB_12_3: NPTH, NPTH, F.Cu at (159.8, 33.3)
- added KiKit_MB_13_1: NPTH, NPTH, F.Cu at (155.9, 38.5)
- added KiKit_MB_13_2: NPTH, NPTH, F.Cu at (154.9, 38.5)
- added KiKit_MB_13_3: NPTH, NPTH, F.Cu at (153.9, 38.5)
- added KiKit_MB_14_1: NPTH, NPTH, F.Cu at (162.8, 27.2)
- added KiKit_MB_14_2: NPTH, NPTH, F.Cu at (162.8, 26.2)
- added KiKit_MB_14_3: NPTH, NPTH, F.Cu at (162.8, 25.2)
- added KiKit_MB_15_1: NPTH, NPTH, F.Cu at (162.8, 33.3)
- added KiKit_MB_15_2: NPTH, NPTH, F.Cu at (162.8, 32.3)
- added KiKit_MB_15_3: NPTH, NPTH, F.Cu at (162.8, 31.3)
- added KiKit_MB_16_1: NPTH, NPTH, F.Cu at (168.7, 38.5)
- added KiKit_MB_16_2: NPTH, NPTH, F.Cu at (167.7, 38.5)
- added KiKit_MB_16_3: NPTH, NPTH, F.Cu at (166.7, 38.5)
- added KiKit_MB_17_1: NPTH, NPTH, F.Cu at (134.2, 46.7)
- added KiKit_MB_17_2: NPTH, NPTH, F.Cu at (134.2, 47.7)
- added KiKit_MB_17_3: NPTH, NPTH, F.Cu at (134.2, 48.7)
- added KiKit_MB_18_1: NPTH, NPTH, F.Cu at (134.2, 52.8)
- added KiKit_MB_18_2: NPTH, NPTH, F.Cu at (134.2, 53.8)
- added KiKit_MB_18_3: NPTH, NPTH, F.Cu at (134.2, 54.8)
- added KiKit_MB_19_1: NPTH, NPTH, F.Cu at (128.3, 41.5)
- added KiKit_MB_19_2: NPTH, NPTH, F.Cu at (129.3, 41.5)
- added KiKit_MB_19_3: NPTH, NPTH, F.Cu at (130.3, 41.5)
- added KiKit_MB_1_1: NPTH, NPTH, F.Cu at (134.2, 25.2)
- added KiKit_MB_1_2: NPTH, NPTH, F.Cu at (134.2, 26.2)
- added KiKit_MB_1_3: NPTH, NPTH, F.Cu at (134.2, 27.2)
- added KiKit_MB_20_1: NPTH, NPTH, F.Cu at (137.2, 48.7)
- added KiKit_MB_20_2: NPTH, NPTH, F.Cu at (137.2, 47.7)
- added KiKit_MB_20_3: NPTH, NPTH, F.Cu at (137.2, 46.7)
- added KiKit_MB_21_1: NPTH, NPTH, F.Cu at (137.2, 54.8)
- added KiKit_MB_21_2: NPTH, NPTH, F.Cu at (137.2, 53.8)
- added KiKit_MB_21_3: NPTH, NPTH, F.Cu at (137.2, 52.8)
- added KiKit_MB_22_1: NPTH, NPTH, F.Cu at (147.0, 46.7)
- added KiKit_MB_22_2: NPTH, NPTH, F.Cu at (147.0, 47.7)
- added KiKit_MB_22_3: NPTH, NPTH, F.Cu at (147.0, 48.7)
- added KiKit_MB_23_1: NPTH, NPTH, F.Cu at (147.0, 52.8)
- added KiKit_MB_23_2: NPTH, NPTH, F.Cu at (147.0, 53.8)
- added KiKit_MB_23_3: NPTH, NPTH, F.Cu at (147.0, 54.8)
- added KiKit_MB_24_1: NPTH, NPTH, F.Cu at (141.1, 41.5)
- added KiKit_MB_24_2: NPTH, NPTH, F.Cu at (142.1, 41.5)
- added KiKit_MB_24_3: NPTH, NPTH, F.Cu at (143.1, 41.5)
- added KiKit_MB_25_1: NPTH, NPTH, F.Cu at (150.0, 48.7)
- added KiKit_MB_25_2: NPTH, NPTH, F.Cu at (150.0, 47.7)
- added KiKit_MB_25_3: NPTH, NPTH, F.Cu at (150.0, 46.7)
- added KiKit_MB_26_1: NPTH, NPTH, F.Cu at (150.0, 54.8)
- added KiKit_MB_26_2: NPTH, NPTH, F.Cu at (150.0, 53.8)
- added KiKit_MB_26_3: NPTH, NPTH, F.Cu at (150.0, 52.8)
- added KiKit_MB_27_1: NPTH, NPTH, F.Cu at (159.8, 46.7)
- added KiKit_MB_27_2: NPTH, NPTH, F.Cu at (159.8, 47.7)
- added KiKit_MB_27_3: NPTH, NPTH, F.Cu at (159.8, 48.7)
- added KiKit_MB_28_1: NPTH, NPTH, F.Cu at (159.8, 52.8)
- added KiKit_MB_28_2: NPTH, NPTH, F.Cu at (159.8, 53.8)
- added KiKit_MB_28_3: NPTH, NPTH, F.Cu at (159.8, 54.8)
- added KiKit_MB_29_1: NPTH, NPTH, F.Cu at (153.9, 41.5)
- added KiKit_MB_29_2: NPTH, NPTH, F.Cu at (154.9, 41.5)
- added KiKit_MB_29_3: NPTH, NPTH, F.Cu at (155.9, 41.5)
- added KiKit_MB_2_1: NPTH, NPTH, F.Cu at (134.2, 31.3)
- added KiKit_MB_2_2: NPTH, NPTH, F.Cu at (134.2, 32.3)
- added KiKit_MB_2_3: NPTH, NPTH, F.Cu at (134.2, 33.3)
- added KiKit_MB_30_1: NPTH, NPTH, F.Cu at (162.8, 48.7)
- added KiKit_MB_30_2: NPTH, NPTH, F.Cu at (162.8, 47.7)
- added KiKit_MB_30_3: NPTH, NPTH, F.Cu at (162.8, 46.7)
- added KiKit_MB_31_1: NPTH, NPTH, F.Cu at (162.8, 54.8)
- added KiKit_MB_31_2: NPTH, NPTH, F.Cu at (162.8, 53.8)
- added KiKit_MB_31_3: NPTH, NPTH, F.Cu at (162.8, 52.8)
- added KiKit_MB_32_1: NPTH, NPTH, F.Cu at (166.7, 41.5)
- added KiKit_MB_32_2: NPTH, NPTH, F.Cu at (167.7, 41.5)
- added KiKit_MB_32_3: NPTH, NPTH, F.Cu at (168.7, 41.5)
- added KiKit_MB_3_1: NPTH, NPTH, F.Cu at (130.3, 38.5)
- added KiKit_MB_3_2: NPTH, NPTH, F.Cu at (129.3, 38.5)
- added KiKit_MB_3_3: NPTH, NPTH, F.Cu at (128.3, 38.5)
- added KiKit_MB_4_1: NPTH, NPTH, F.Cu at (137.2, 27.2)
- added KiKit_MB_4_2: NPTH, NPTH, F.Cu at (137.2, 26.2)
- added KiKit_MB_4_3: NPTH, NPTH, F.Cu at (137.2, 25.2)
- added KiKit_MB_5_1: NPTH, NPTH, F.Cu at (137.2, 33.3)
- added KiKit_MB_5_2: NPTH, NPTH, F.Cu at (137.2, 32.3)
- added KiKit_MB_5_3: NPTH, NPTH, F.Cu at (137.2, 31.3)
- added KiKit_MB_6_1: NPTH, NPTH, F.Cu at (147.0, 25.2)
- added KiKit_MB_6_2: NPTH, NPTH, F.Cu at (147.0, 26.2)
- added KiKit_MB_6_3: NPTH, NPTH, F.Cu at (147.0, 27.2)
- added KiKit_MB_7_1: NPTH, NPTH, F.Cu at (147.0, 31.3)
- added KiKit_MB_7_2: NPTH, NPTH, F.Cu at (147.0, 32.3)
- added KiKit_MB_7_3: NPTH, NPTH, F.Cu at (147.0, 33.3)
- added KiKit_MB_8_1: NPTH, NPTH, F.Cu at (143.1, 38.5)
- added KiKit_MB_8_2: NPTH, NPTH, F.Cu at (142.1, 38.5)
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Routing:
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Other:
- board size 45.2 x 39 mm -> 48.2 x 40 mm
- board text added: "Ru-Pirie"
